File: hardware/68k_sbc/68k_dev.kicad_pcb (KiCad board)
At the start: 2 copper layers, 186.7 x 144.8 mm, 72 parts, among them IC1 DS1813-10+T&R, J1 640456-3, J2 Passive_Bus_ISA_16bit, J3 Conn_02x20_Odd_Even, J4 JTAG, J5 Barrel_Jack, U1 68000D, U10 CY7C1049D, U11 CY7C1049D, U12 CY7C1049D, U13 CY7C1049D, U14 16550, U15 TXS0108EPW, U2 M27C1024, U3 EPM7128SLC84-15N, U5 AMS1117-3.3, U6 CY7C1049D, U7 CY7C1049D, U8 CY7C1049D, U9 CY7C1049D, X1 CXO_DIP8, X2 CXO_DIP14

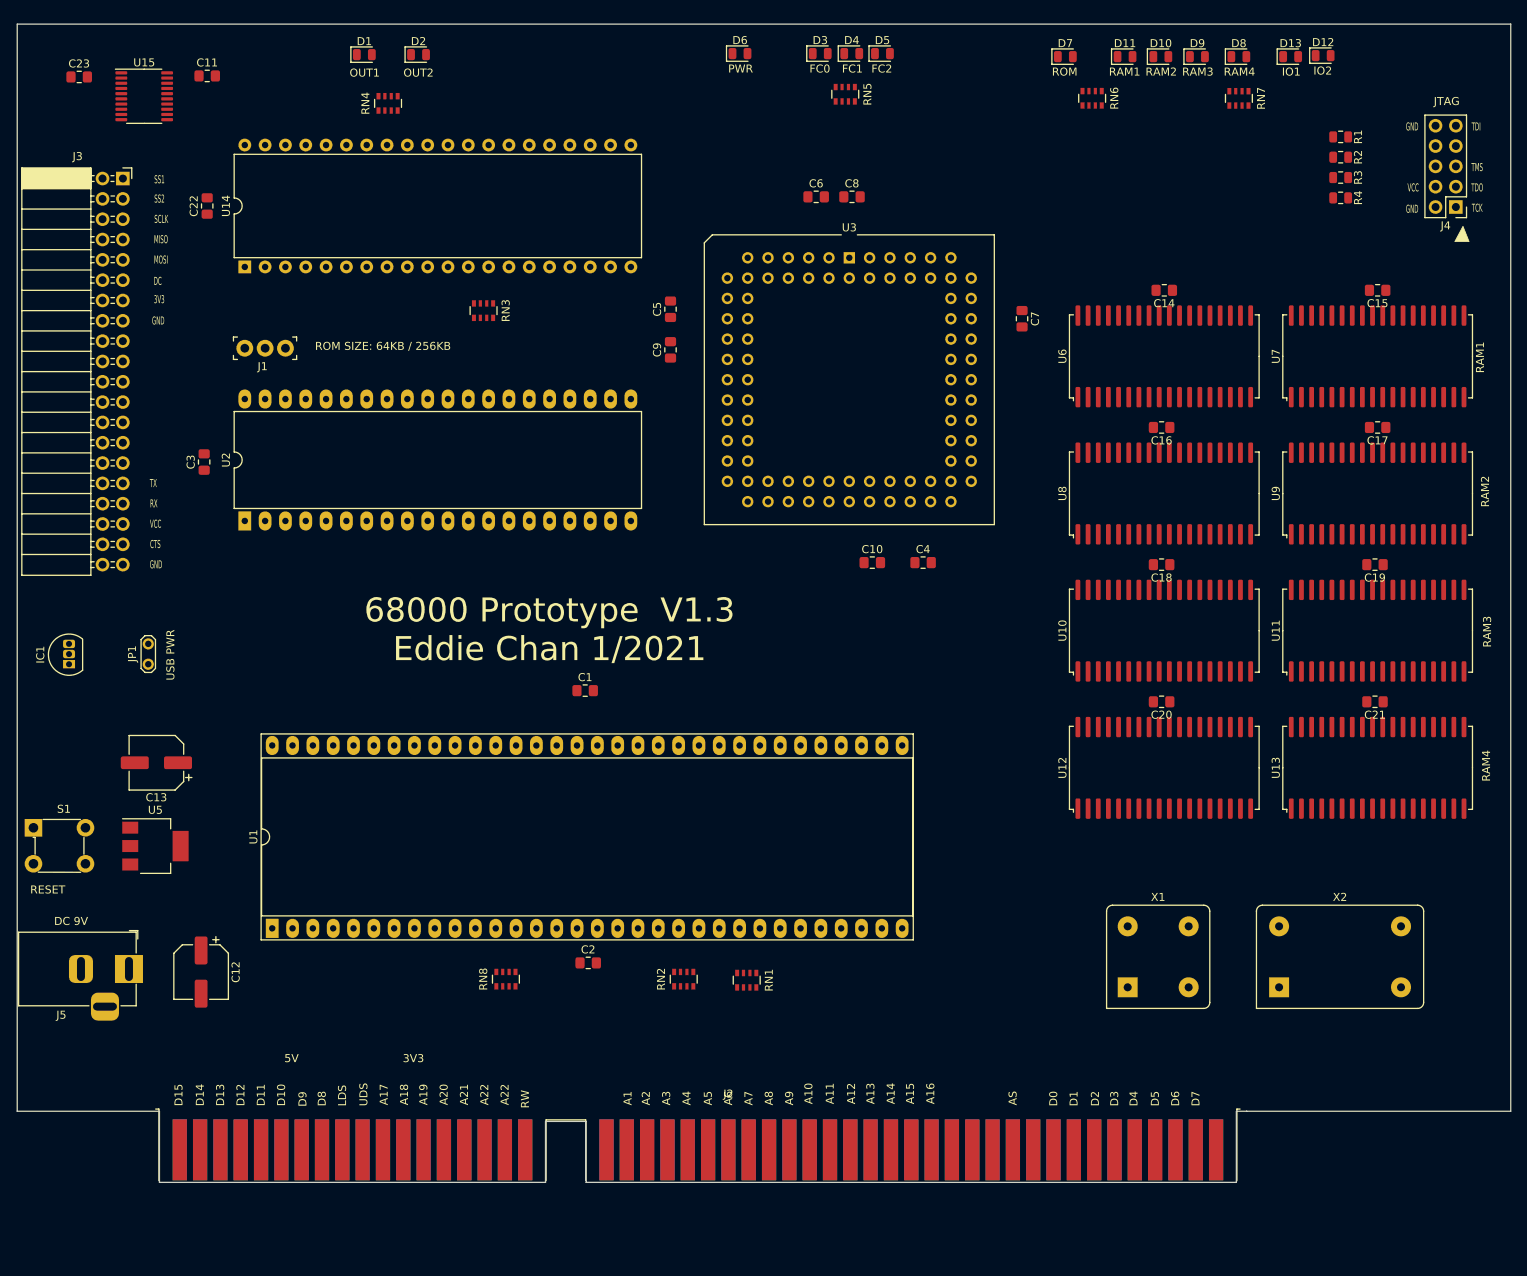
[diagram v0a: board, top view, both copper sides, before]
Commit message: lib refactor
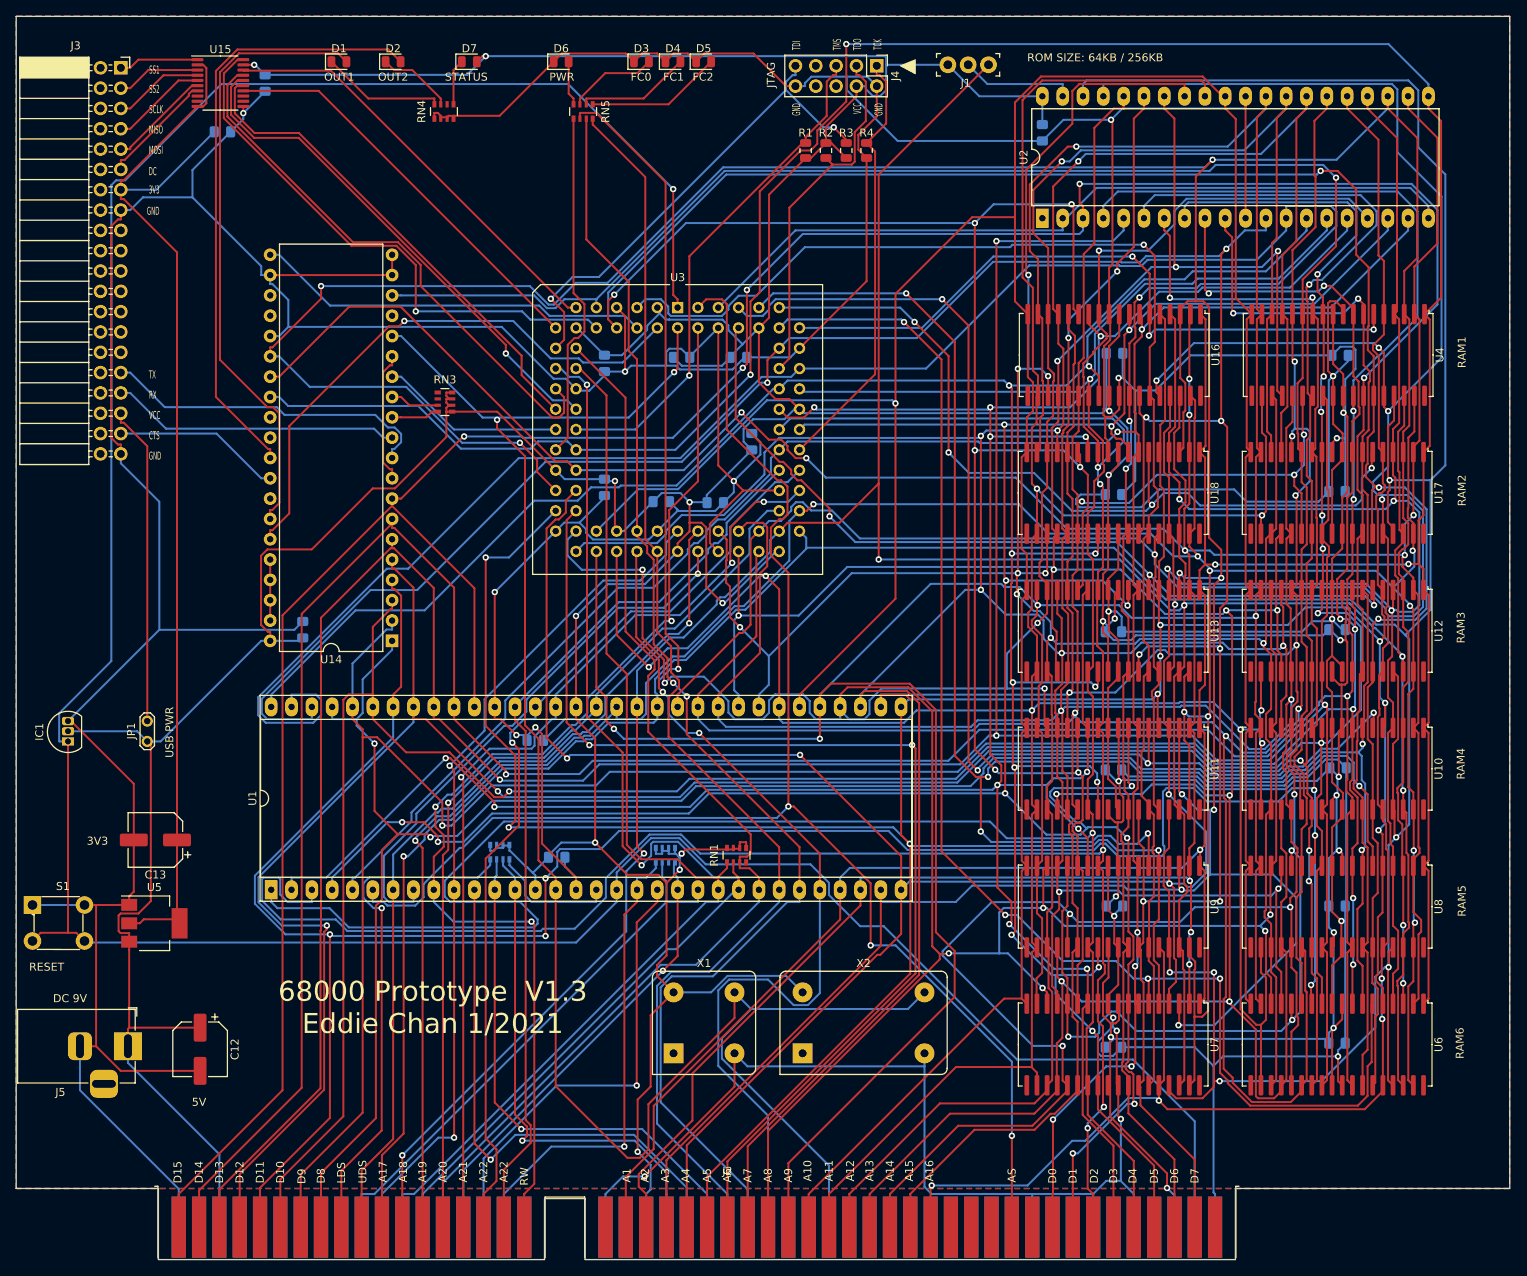
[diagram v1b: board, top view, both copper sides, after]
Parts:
- removed D10, D11, D12, D13, D8, D9: LED, LED_SMD:LED_0805_2012Metric
- removed RN6, RN7: 470, Resistor_SMD:R_Array_Convex_4x0603
- added C24: 100nF, Capacitor_SMD:C_0805_2012Metric_Pad1.15x1.40mm_HandSolder, B.Cu at (153.5, 72.8)
- added C25: 100nF, Capacitor_SMD:C_0805_2012Metric_Pad1.15x1.40mm_HandSolder, B.Cu at (153.5, 89.9)
- added C26: 100nF, Capacitor_SMD:C_0805_2012Metric_Pad1.15x1.40mm_HandSolder, B.Cu at (153.7, 55.1)
- added C27: 100nF, Capacitor_SMD:C_0805_2012Metric_Pad1.15x1.40mm_HandSolder, B.Cu at (181.5, 72.4)
- added U16: CY7C1049D, KiCad_Libraries:SOJ-36_10.16x23.49mm_P1.27mm_sram, F.Cu at (153.6, 55.3)
- added U17: CY7C1049D, KiCad_Libraries:SOJ-36_10.16x23.49mm_P1.27mm_sram, F.Cu at (181.5, 72.6)
- added U18: CY7C1049D, KiCad_Libraries:SOJ-36_10.16x23.49mm_P1.27mm_sram, F.Cu at (153.5, 72.6)
- added U4: CY7C1049D, KiCad_Libraries:SOJ-36_10.16x23.49mm_P1.27mm_sram, F.Cu at (181.6, 55.3)
- C1, C10, C11, C14, C15, C16, C17, C18, C19, C2, C20, C21, C22, C23, C3, C4, C5, C6, C7, C8, C9, RN2, RN8: moved to B.Cu
- moved C3 112.6 mm to (144.7, 27.6), turned to 270 degrees
- moved U2 106.6 mm to (144.7, 38.2)
- moved J1 94.8 mm to (137.9, 19.1)
- moved U7 92.2 mm to (153.5, 141.5), turned to 270 degrees
- moved U6 88.7 mm to (181.5, 141.5), turned to 270 degrees
- moved C16 77.7 mm to (153.5, 141.9), turned to 0 degrees
- moved C17 77.1 mm to (181.5, 141.4), turned to 0 degrees
- moved J4 74.5 mm to (124.0, 19.2), turned to 270 degrees
- moved D7 74.5 mm to (73.0, 18.7)
- moved R1 66.9 mm to (115.1, 29.8), turned to 90 degrees
- moved R2 64.3 mm to (117.6, 29.8), turned to 270 degrees
- moved R3 61.9 mm to (120.1, 29.8), turned to 90 degrees
- moved U9 61.3 mm to (153.5, 124.3), turned to 270 degrees
- moved X2 60.1 mm to (114.7, 142.6)
- moved R4 59.6 mm to (122.7, 29.8), turned to 270 degrees
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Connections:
- D7 pad 1: GND -> Net-(D7-Pad1)
- D7 pad 2: Net-(D7-Pad2) -> VCC
- J2 pad 13: IO_SEL1 -> Net-(J2-Pad13)
- J2 pad 14: IO_SEL2 -> Net-(J2-Pad14)
- J2 pad 15: RAM1_SEL -> Net-(J2-Pad15)
- J2 pad 16: RAM2_SEL -> Net-(J2-Pad16)
- J2 pad 17: RAM3_SEL -> Net-(J2-Pad17)
- J2 pad 18: RAM4_SEL -> Net-(J2-Pad18)
- J2 pad 19: ROM_SEL -> Net-(J2-Pad19)
- J2 pad 4: RST_H -> Net-(J2-Pad4)
- J2 pad 72: RDL -> Net-(J2-Pad72)
- J2 pad 73: RDU -> Net-(J2-Pad73)
- J2 pad 74: WRL -> Net-(J2-Pad74)
- J2 pad 75: WRU -> Net-(J2-Pad75)
- J2 pad 76: IRQ1 -> Net-(J2-Pad76)
- J2 pad 77: IRQ2 -> Net-(J2-Pad77)
- J2 pad 9: +3V3 -> Net-(J2-Pad9)
- RN1 pad 1: IPL0 -> IPL2
- RN1 pad 3: IPL2 -> IPL0
- RN2 pad 2: DTACK -> Net-(RN2-Pad2)
- RN2 pad 4: BR -> VMA
- RN4 pad 5: Net-(RN4-Pad5) -> Net-(D7-Pad1)
- RN4 pad 7: Net-(D1-Pad1) -> Net-(D2-Pad1)
- RN4 pad 8: Net-(D2-Pad1) -> Net-(D1-Pad1)
- RN5 pad 1: Net-(D3-Pad2) -> Net-(D5-Pad2)
- RN5 pad 3: Net-(D5-Pad2) -> Net-(D3-Pad2)
- RN5 pad 5: VCC -> STATUS
- RN5 pad 6: FC2 -> FC0
- RN5 pad 8: FC0 -> FC2
- RN8 pad 1: BGACK -> Net-(RN8-Pad1)
- RN8 pad 2: VMA -> BR
- RN8 pad 3: Net-(RN8-Pad3) -> BGACK
- RN8 pad 4: Net-(RN8-Pad4) -> DTACK
- U1 pad 17: Net-(RN1-Pad4) -> Net-(RN8-Pad1)
- U14 pad 30: IRQ1 -> Net-(U14-Pad30)
- U3 pad 22: IRQ1 -> IO_SEL1
- U3 pad 24: IRQ2 -> STATUS
- U3 pad 74: IO_SEL1 -> RAM5_SEL
- U3 pad 75: IO_SEL2 -> RAM6_SEL
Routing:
- net GND: track 0.00 -> 1228.2 mm, vias 0 -> 19
- net VCC: track 0.00 -> 1070.5 mm, vias 0 -> 25
- net A3: track 0.00 -> 593.9 mm, vias 0 -> 11
- net A17: track 0.00 -> 536.0 mm, vias 0 -> 8
- net A1: track 0.00 -> 525.3 mm, vias 0 -> 5
- net A16: track 0.00 -> 472.6 mm, vias 0 -> 9
- net A7: track 0.00 -> 471.9 mm, vias 0 -> 8
- net A2: track 0.00 -> 469.3 mm, vias 0 -> 10
- net A5: track 0.00 -> 464.2 mm, vias 0 -> 10
- net A9: track 0.00 -> 449.3 mm, vias 0 -> 5
- net A4: track 0.00 -> 447.2 mm, vias 0 -> 8
- net A8: track 0.00 -> 446.9 mm, vias 0 -> 10
- net A6: track 0.00 -> 445.8 mm, vias 0 -> 11
- net A18: track 0.00 -> 443.0 mm, vias 0 -> 6
- net A11: track 0.00 -> 426.3 mm, vias 0 -> 8
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- added copper zone on B.Cu, net GND
- added copper zone on F.Cu, net GND
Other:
- board size 186.7 x 144.8 mm -> 186.7 x 155.4 mm
- board text added: "RAM5"
- board text added: "RAM6"
- board text added: "STATUS"
- board text removed: "IO1"
- board text removed: "IO1_SEL"
- board text removed: "IO2"
- board text removed: "IO2_SEL"
- board text removed: "RAM1_SEL"
- board text removed: "RAM2_SEL"
- board text removed: "RAM3_SEL"
- board text removed: "RAM4_SEL"
- board text removed: "ROM"
- board text removed: "ROM_SEL"

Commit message: updates
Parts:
- removed C11: 100nF, Capacitor_SMD:C_0805_2012Metric_Pad1.15x1.40mm_HandSolder
- removed X1: CXO_DIP8, Oscillator:Oscillator_DIP-8_LargePads
- added C28: 100nF, Capacitor_SMD:C_0805_2012Metric_Pad1.15x1.40mm_HandSolder, B.Cu at (227.3, 146.9)
- added C29: 100nF, Capacitor_SMD:C_0805_2012Metric_Pad1.15x1.40mm_HandSolder, B.Cu at (126.0, 129.4)
- added C30: 100nF, Capacitor_SMD:C_0805_2012Metric_Pad1.15x1.40mm_HandSolder, B.Cu at (160.0, 123.4)
- added C31: 100nF, Capacitor_SMD:C_0805_2012Metric_Pad1.15x1.40mm_HandSolder, B.Cu at (196.3, 124.0)
- added C32: 100nF, Capacitor_SMD:C_0805_2012Metric_Pad1.15x1.40mm_HandSolder, F.Cu at (138.7, 123.6)
- added C33: 100nF, Capacitor_SMD:C_0805_2012Metric_Pad1.15x1.40mm_HandSolder, B.Cu at (113.0, 13.8)
- added C34: 100nF, Capacitor_SMD:C_0805_2012Metric_Pad1.15x1.40mm_HandSolder, B.Cu at (100.8, 13.8)
- added G***: LOGO, logos:twitter, F.Cu at (139.3, 132.8)
- added U20: 74LS244, Package_SO:SSOP-20_5.3x7.2mm_P0.65mm, F.Cu at (180.2, 128.8)
- added U21: 74LS244, Package_SO:SSOP-20_5.3x7.2mm_P0.65mm, B.Cu at (138.7, 128.7)
- added U22: 74LS244, Package_SO:SSOP-20_5.3x7.2mm_P0.65mm, F.Cu at (196.3, 128.9)
- added U23: SN74LVC245AN, KiCad_Libraries:SOIC127P1032X265-20N, F.Cu at (219.5, 147.1)
- added U24: SN74LVC245AN, KiCad_Libraries:SOIC127P1032X265-20N, F.Cu at (118.0, 129.3)
- added U25: TXS0108EPW, Package_SO:TSSOP-20_4.4x6.5mm_P0.65mm, F.Cu at (106.9, 18.3)
- RN1, RN3: moved to B.Cu
- U15: value TXS0108EPW -> 74LS244; footprint Package_SO:TSSOP-20_4.4x6.5mm_P0.65mm -> Package_SO:SSOP-20_5.3x7.2mm_P0.65mm
- moved C23 168.4 mm to (180.2, 123.8), turned to 180 degrees
- moved U15 159.7 mm to (160.1, 128.7)
- moved X2 119.4 mm to (191.5, 51.2), turned to 270 degrees
- moved RN4 72.9 mm to (142.6, 20.1)
- moved C22 72.6 mm to (121.9, 69.3)
- moved U14 72.6 mm to (133.1, 70.7)
- moved C14 70.1 mm to (251.1, 44.5), turned to 0 degrees
- moved C15 70.1 mm to (250.7, 78.7)
- moved C16 70.1 mm to (222.7, 130.9)
- moved C17 70.1 mm to (250.7, 130.4)
- moved C18 70.1 mm to (222.9, 113.3)
- moved C19 70.1 mm to (250.7, 113.3)
- moved C20 70.1 mm to (222.8, 96.3)
- moved C24 70.1 mm to (222.8, 61.8)
- moved C25 70.1 mm to (222.8, 79.0)
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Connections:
- C23 pad 1: +3V3 -> VCC
- J2 pad 20: CPU_CLK -> BUS_CPU_CLK
- J2 pad 23: FC0 -> BUS_FC0
- J2 pad 24: FC1 -> BUS_FC1
- J2 pad 25: FC2 -> BUS_FC2
- J2 pad 27: BG -> BUS_BG
- J2 pad 33: D7 -> BUS_D7
- J2 pad 34: D6 -> BUS_D6
- J2 pad 35: D5 -> BUS_D5
- J2 pad 36: D4 -> BUS_D4
- J2 pad 37: D3 -> BUS_D3
- J2 pad 38: D2 -> BUS_D2
- J2 pad 39: D1 -> BUS_D1
- J2 pad 40: D0 -> BUS_D0
- J2 pad 42: AS -> BUS_AS
- J2 pad 46: A16 -> BUS_A16
- J2 pad 47: A15 -> BUS_A15
- J2 pad 48: A14 -> BUS_A14
- J2 pad 49: A13 -> BUS_A13
- J2 pad 50: A12 -> BUS_A12
- J2 pad 51: A11 -> BUS_A11
- J2 pad 52: A10 -> BUS_A10
- J2 pad 53: A9 -> BUS_A9
- J2 pad 54: A8 -> BUS_A8
- J2 pad 55: A7 -> BUS_A7
- J2 pad 56: A6 -> BUS_A6
- J2 pad 57: A5 -> BUS_A5
- J2 pad 58: A4 -> BUS_A4
- J2 pad 59: A3 -> BUS_A3
- J2 pad 60: A2 -> BUS_A2
- J2 pad 61: A1 -> BUS_A1
- J2 pad 81: RW -> BUS_RW
- J2 pad 82: A23 -> BUS_A23
- J2 pad 83: A22 -> BUS_A22
- J2 pad 84: A21 -> BUS_A21
- J2 pad 85: A20 -> BUS_A20
- J2 pad 86: A19 -> BUS_A19
- J2 pad 87: A18 -> BUS_A18
- J2 pad 88: A17 -> BUS_A17
- J2 pad 89: UDS -> BUS_UDS
- J2 pad 90: LDS -> BUS_LDS
- J2 pad 91: D8 -> BUS_D8
- J2 pad 92: D9 -> BUS_D9
- J2 pad 93: D10 -> BUS_D10
- J2 pad 94: D11 -> BUS_D11
- J2 pad 95: D12 -> BUS_D12
- J2 pad 96: D13 -> BUS_D13
- J2 pad 97: D14 -> BUS_D14
- J2 pad 98: D15 -> BUS_D15
- U15 pad 1: Net-(J3-Pad1) -> GND
- U15 pad 10: +3V3 -> GND
- U15 pad 11: GND -> A20
- U15 pad 12: Net-(U15-Pad12) -> BUS_A21
- U15 pad 13: Net-(U15-Pad13) -> A19
- U15 pad 14: DC -> BUS_A22
- U15 pad 15: MOSI -> A18
- U15 pad 16: MISO -> BUS_A23
- U15 pad 17: SCLK -> A17
- U15 pad 18: SS2 -> BUS_RW
- U15 pad 19: VCC -> GND
- U15 pad 2: +3V3 -> RW
- U15 pad 20: SS1 -> VCC
- U15 pad 3: Net-(J3-Pad3) -> BUS_A17
- U15 pad 4: Net-(J3-Pad5) -> A23
- U15 pad 5: Net-(J3-Pad7) -> BUS_A18
- U15 pad 6: Net-(J3-Pad9) -> A22
- U15 pad 7: Net-(J3-Pad11) -> BUS_A19
- U15 pad 8: Net-(U15-Pad8) -> A21
- U15 pad 9: Net-(U15-Pad9) -> BUS_A20
- U3 pad 31: A6 -> A18
- U3 pad 33: A7 -> A19
- U3 pad 34: A8 -> A20
- U3 pad 35: A9 -> A21
- U3 pad 36: A10 -> A22
- U3 pad 37: A11 -> A23
- U3 pad 48: A12 -> IPL2
- U3 pad 49: A13 -> IPL1
- U3 pad 50: A14 -> IPL0
- U3 pad 51: A15 -> BUS_DIR_CTRL
- U3 pad 52: A16 -> D0
- U3 pad 54: A17 -> D1
- U3 pad 55: A18 -> D2
- U3 pad 56: A19 -> D3
- U3 pad 57: A20 -> D4
- U3 pad 58: A21 -> D5
- U3 pad 60: A22 -> D6
- U3 pad 61: A23 -> D7
- U3 pad 63: D0 -> D8
- U3 pad 64: D1 -> D9
- U3 pad 65: D2 -> D10
- U3 pad 67: D3 -> D11
- U3 pad 68: D4 -> D12
- U3 pad 69: D5 -> D13
- U3 pad 70: D6 -> D14
- U3 pad 73: D7 -> D15
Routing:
- net GND: track 1228.2 -> 1460.2 mm, vias 19 -> 28
- net BUS_DIR_CTRL: track 0.00 -> 206.3 mm, vias 0 -> 1
- net RAM4_SEL: track 105.7 -> 242.0 mm, vias 3 -> 5
- net A8: track 446.9 -> 316.0 mm, vias 10 -> 3
- net A7: track 471.9 -> 357.6 mm, vias 8 -> 9
- net BUS_CPU_CLK: track 0.00 -> 110.4 mm, vias 0 -> 2
- net A10: track 422.9 -> 320.7 mm, vias 1 -> 2
- net A9: track 449.3 -> 349.5 mm, vias 5 -> 7
- net A17: track 536.0 -> 446.9 mm, vias 8 -> 6
- net A6: track 445.8 -> 362.1 mm, vias 11 -> 6
- net A1: track 525.3 -> 441.8 mm, vias 5 -> 4
- net RW: track 143.4 -> 225.8 mm, vias 3 -> 5
- net AS: track 198.7 -> 117.3 mm, vias 3 -> 5
- net BUS_AS: track 0.00 -> 80.7 mm, vias 0 -> 3
- net D13: track 408.7 -> 330.7 mm, vias 4 -> 7
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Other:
- board size 186.7 x 155.4 mm -> 190.5 x 158.4 mm
- board text added: "68000 Prototype V1.4 Eddie Chan 02/2021"
- board text removed: "68000 Prototype V1.3 Eddie Chan 1/2021"
